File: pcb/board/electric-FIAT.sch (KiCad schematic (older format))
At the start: 0 parts

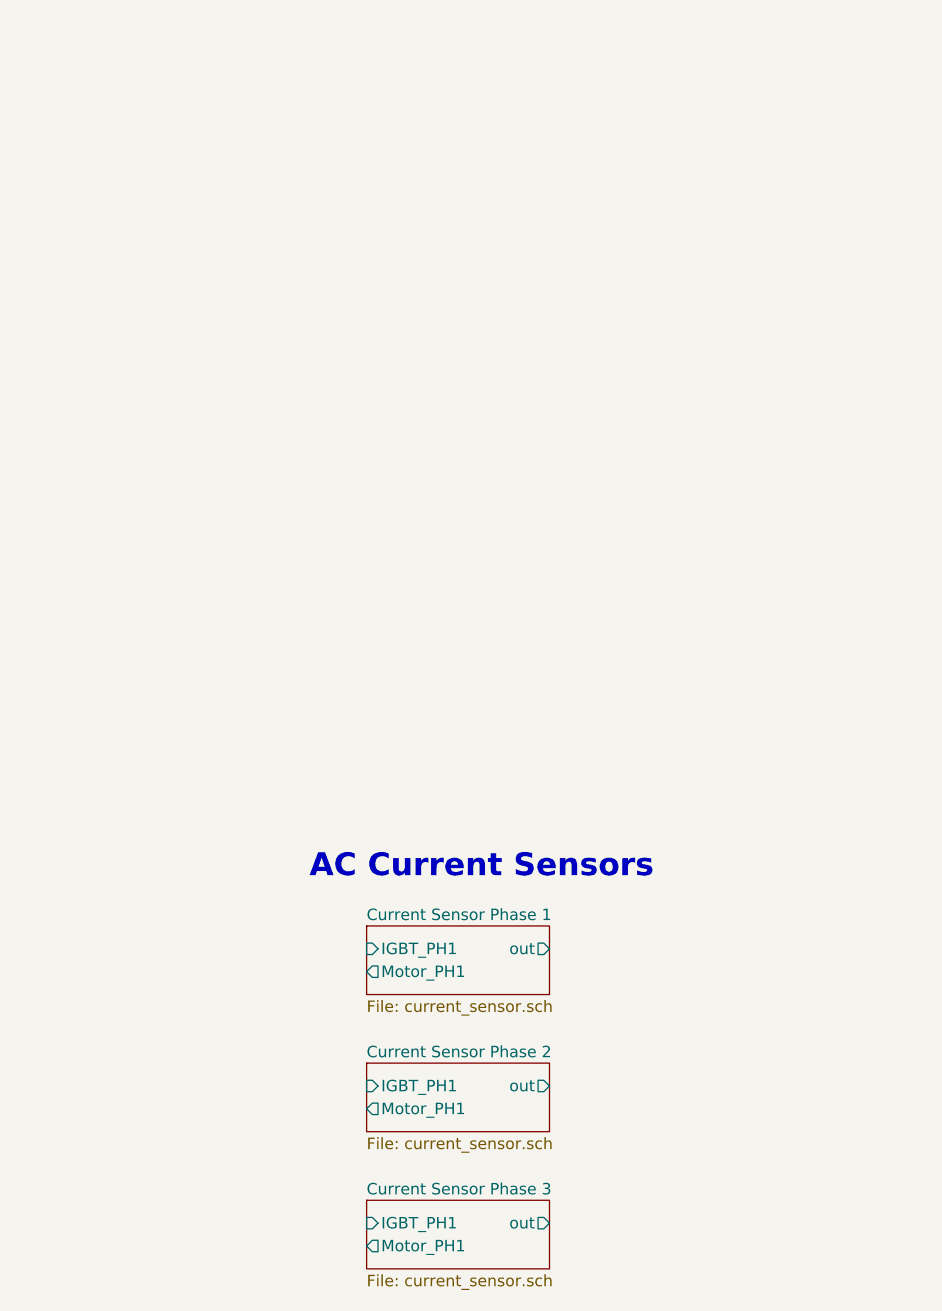
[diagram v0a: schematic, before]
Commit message: Thermistor
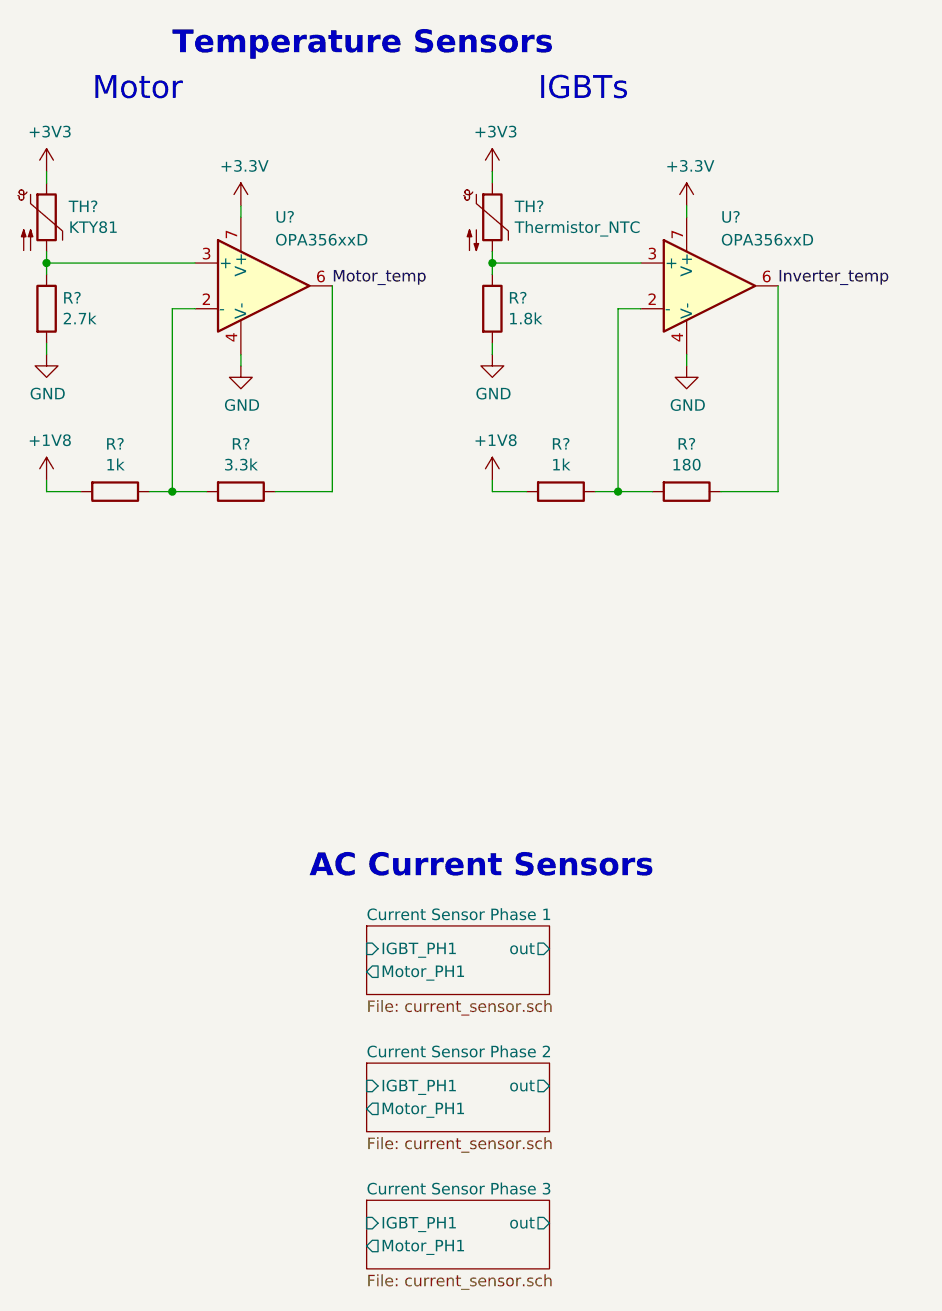
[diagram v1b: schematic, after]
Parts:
- added R?: 3.3k, symbol Device:R
- added R? (x2): 1k, symbol Device:R
- added R?: 2.7k, symbol Device:R
- added R?: 180, symbol Device:R
- added R?: 1.8k, symbol Device:R
- added TH?: KTY81, symbol Sensor_Temperature:KTY81
- added TH?: Thermistor_NTC, symbol Device:Thermistor_NTC
- added U? (x2): OPA356xxD, Package_SO:SOIC-8_3.9x4.9mm_P1.27mm, symbol Amplifier_Operational:OPA356xxD
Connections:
- new net: R?.1, R?.2, U?.2 (-) (x2)
- new net: R?.1, TH?.2, U?.3 (+) (x2)
- new net +1V8: R?.2, R?.2
- new net +3V3: TH?.1, TH?.1, U?.7 (V+), U?.7 (V+)
- new net GND: R?.2, R?.2, U?.4 (V-), U?.4 (V-)
- new net Inverter_temp: R?.1, U?.6
- new net Motor_temp: R?.1, U?.6
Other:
- note added: "IGBTs"
- note added: "Motor"
- note added: "Temperature Sensors"
